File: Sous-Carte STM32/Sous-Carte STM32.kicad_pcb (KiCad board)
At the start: 2 copper layers, 117.5 x 123 mm, 34 parts, among them J1 RJ45, P1 CONN_25X2, P2 CONN_25X2, P3 CONN_4, P5 CONN_25X2, P6 CONN_2, P7 CONN_2, P8 CONN_2

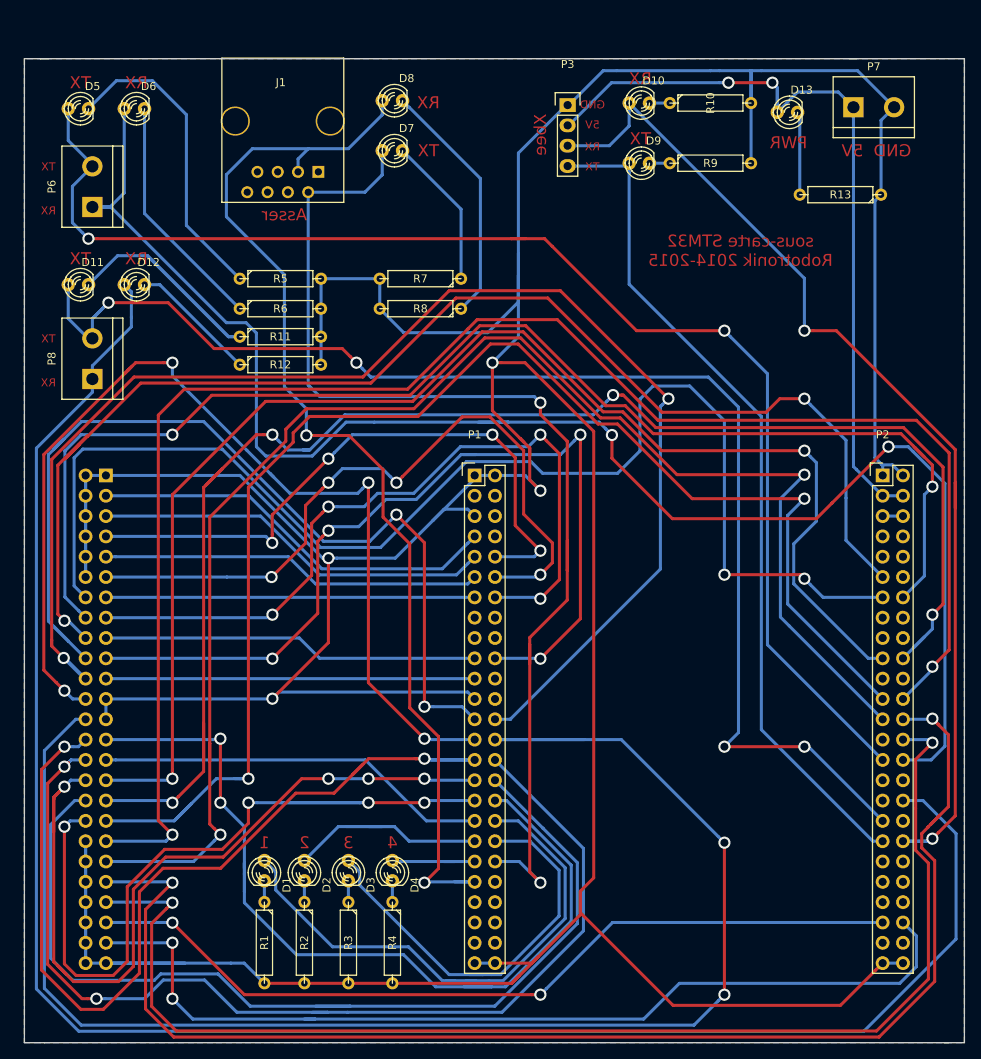
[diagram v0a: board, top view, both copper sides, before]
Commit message: bougé la carte
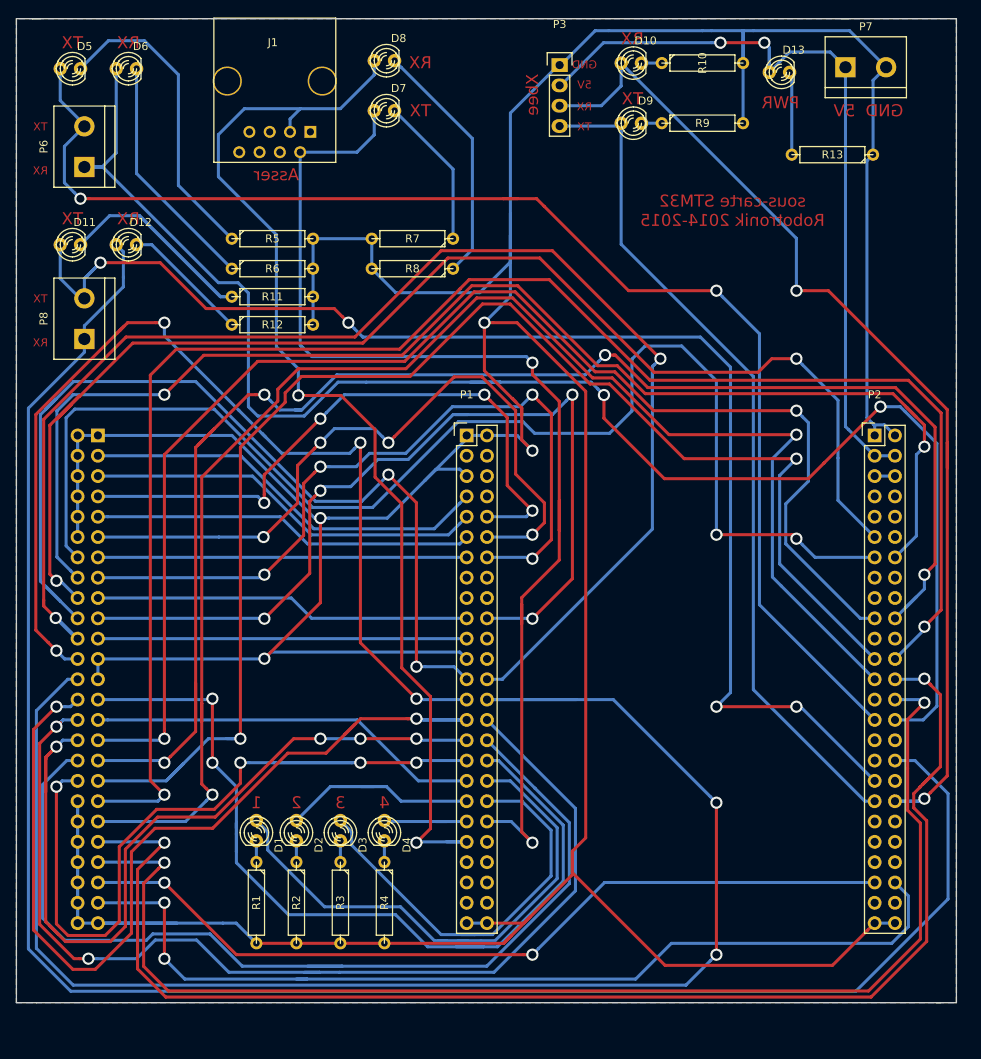
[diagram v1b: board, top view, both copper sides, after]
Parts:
- moved D1 5.10 mm to (116.5, 142.5)
- moved D10 5.10 mm to (163.4, 46.5)
- moved D11 5.10 mm to (93.2, 69.2)
- moved D12 5.10 mm to (100.2, 69.2)
- moved D13 5.10 mm to (181.9, 47.7)
- moved D2 5.10 mm to (121.5, 142.5)
- moved D3 5.10 mm to (127.0, 142.5)
- moved D4 5.10 mm to (132.5, 142.5)
- moved D5 5.10 mm to (93.2, 47.2)
- moved D6 5.10 mm to (100.2, 47.2)
- moved D7 5.10 mm to (132.5, 52.5)
- moved D8 5.10 mm to (132.5, 46.2)
- moved D9 5.10 mm to (163.4, 54.1)
- moved J1 5.10 mm to (118.8, 48.8)
- moved P1 5.10 mm to (142.8, 93.1)
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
